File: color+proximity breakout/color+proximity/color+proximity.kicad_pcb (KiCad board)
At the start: 2 copper layers, 72.2 x 21 mm, 59 parts, among them IC1 VL53L4CDV0DH_1, IC2 ISL29125IROZ-T7, J1 RJ12_Shielded, J2 Conn_01x04, J3 Conn_01x06, J8 RJ12_Shielded, J9 Conn_01x06, SW5 SW_Coded_SH-7050, U1 PCA9615DP, U2 LTC4316, U5 TPS73101DBV, U6 ICM-20602

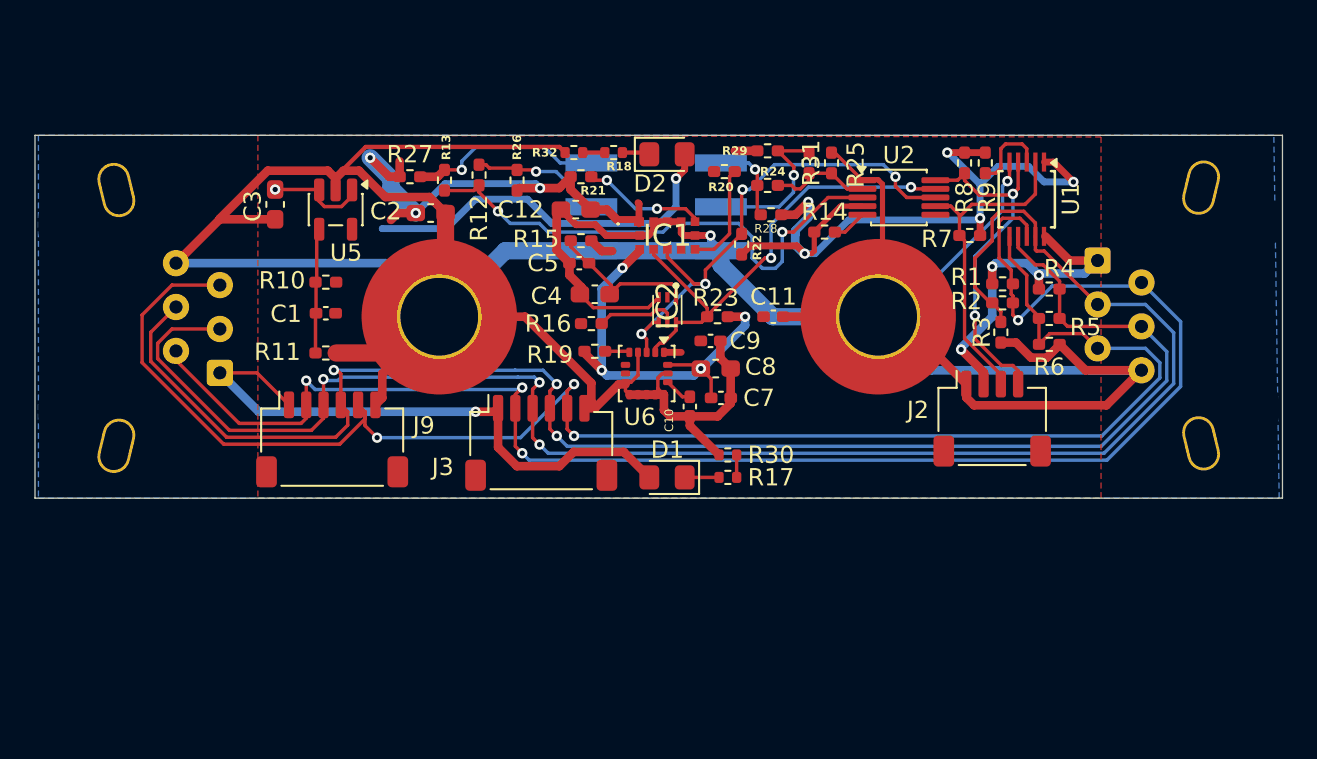
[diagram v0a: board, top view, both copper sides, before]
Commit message: not my finest work but at least it works (i hope)
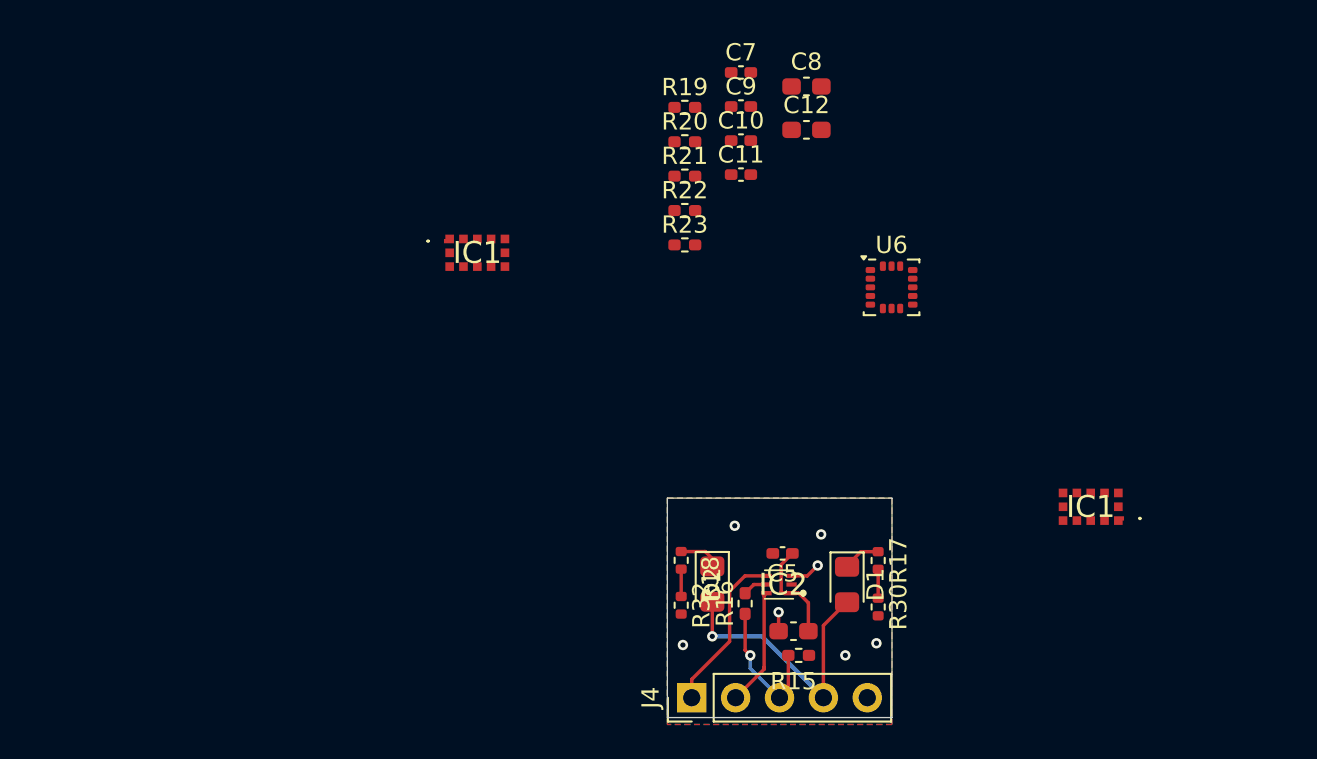
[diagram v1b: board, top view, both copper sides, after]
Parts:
- removed C1: 1n, Capacitor_SMD:C_0402_1005Metric_Pad0.74x0.62mm_HandSolder
- removed C2, C3: 1u, Capacitor_SMD:C_0603_1608Metric_Pad1.08x0.95mm_HandSolder
- removed H1, H2: MountingHole_Pad, MountingHole:MountingHole_4.5mm_Pad_TopOnly
- removed J1, J8: RJ12_Shielded, RJ12_Pin_Connector:RJ12_Pin_Connector
- removed J2: Conn_01x04, Connector_JST:JST_SH_SM04B-SRSS-TB_1x04-1MP_P1.00mm_Horizontal
- removed J3, J9: Conn_01x06, Connector_JST:JST_SH_SM06B-SRSS-TB_1x06-1MP_P1.00mm_Horizontal
- removed R1, R3, R4, R6: 600, Resistor_SMD:R_0402_1005Metric_Pad0.72x0.64mm_HandSolder
- removed R10: 52k, Resistor_SMD:R_0402_1005Metric_Pad0.72x0.64mm_HandSolder
- removed R11: 30k, Resistor_SMD:R_0402_1005Metric_Pad0.72x0.64mm_HandSolder
- removed R12, R24: 400k, Resistor_SMD:R_0402_1005Metric_Pad0.72x0.64mm_HandSolder
- removed R13: 750k, Resistor_SMD:R_0402_1005Metric_Pad0.72x0.64mm_HandSolder
- removed R14, R26, R27, R9: 10k, Resistor_SMD:R_0402_1005Metric_Pad0.72x0.64mm_HandSolder
- removed R2, R5: 120, Resistor_SMD:R_0402_1005Metric_Pad0.72x0.64mm_HandSolder
- removed R25: 780k, Resistor_SMD:R_0402_1005Metric_Pad0.72x0.64mm_HandSolder
- removed R28: 80k, Resistor_SMD:R_0402_1005Metric_Pad0.72x0.64mm_HandSolder
- removed R29: 40k, Resistor_SMD:R_0402_1005Metric_Pad0.72x0.64mm_HandSolder
- removed R31: 260k, Resistor_SMD:R_0402_1005Metric_Pad0.72x0.64mm_HandSolder
- removed R7, R8: 4.7k, Resistor_SMD:R_0402_1005Metric_Pad0.72x0.64mm_HandSolder
- removed SW5: SW_Coded_SH-7050, RJ12_Pin_Connector:Rotary_Switch_16_pos
- removed U1: PCA9615DP, Package_SO:TSSOP-10_3x3mm_P0.5mm
- removed U2: LTC4316, Package_SO:MSOP-10_3x3mm_P0.5mm
- removed U5: TPS73101DBV, Package_TO_SOT_SMD:SOT-23-5
- added IC1: VL53L4CDV0DH_1, VL53L4CD:VL53L4CDV0DH1, F.Cu at (126.2, 105.3)
- added J4: Conn_01x05, Connector_PinHeader_2.54mm:PinHeader_1x05_P2.54mm_Vertical, F.Cu at (103.1, 116.3)
- moved R15 27.1 mm to (109.3, 113.9), turned to 180 degrees
- moved R32 26.9 mm to (102.5, 111.0), turned to -90 degrees
- moved D2 25.0 mm to (104.3, 109.8), turned to -90 degrees
- moved R18 23.9 mm to (102.5, 108.4), turned to -90 degrees
- moved C4 22.6 mm to (109.0, 112.5)
- moved C5 20.5 mm to (108.4, 108.0)
- moved C7 18.9 mm to (106.0, 80.2)
- moved R16 18.5 mm to (106.2, 110.9), turned to 90 degrees
- moved IC2 17.2 mm to (108.2, 109.8), turned to 180 degrees
- moved C8 17.1 mm to (109.8, 81.0)
- moved C10 15.7 mm to (106.0, 84.1), turned to 0 degrees
- moved R19 15.0 mm to (102.7, 82.2)
- moved U6 15.0 mm to (114.7, 92.6), turned to 0 degrees
- moved C12 14.1 mm to (109.8, 83.5), turned to 0 degrees
- moved C9 13.7 mm to (106.0, 82.1)
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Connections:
- IC2 pad 4: /Sensors/sda -> /sda
- IC2 pad 6: /Sensors/scl -> /scl
- R22 pad 2: /Sensors/sda -> /sda
- R23 pad 2: /Sensors/scl -> /scl
- U6 pad 2: /Sensors/scl -> /scl
- U6 pad 3: /Sensors/sda -> /sda
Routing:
- net GND: track 236.8 -> 2.92 mm, vias 2 -> 7
- net Net-(J3-Pin_3): track 98.5 -> 0.00 mm, vias 3 -> 0
- net Net-(J3-Pin_5): track 93.3 -> 0.00 mm, vias 3 -> 0
- net Net-(J3-Pin_2): track 92.6 -> 0.00 mm, vias 4 -> 0
- net Net-(J3-Pin_4): track 89.3 -> 0.00 mm, vias 3 -> 0
- net +3.3V: track 97.1 -> 8.34 mm, vias 12 -> 1
- net +5V: track 82.4 -> 16.0 mm, vias 6 -> 1
- net Net-(U2-XORL): track 30.4 -> 0.00 mm, vias 2 -> 0
- net /Sensors/sda: track 29.9 -> 0.00 mm, vias 4 -> 0
- net /Sensors/scl: track 27.0 -> 0.00 mm, vias 2 -> 0
- net Net-(J2-Pin_4): track 20.8 -> 0.00 mm, vias 2 -> 0
- net Net-(J2-Pin_3): track 19.3 -> 0.00 mm
- net Net-(R13-Pad1): track 11.3 -> 0.00 mm, vias 1 -> 0
- net /sda: track 0.00 -> 9.57 mm
- net Net-(R25-Pad1): track 9.18 -> 0.00 mm, vias 1 -> 0
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- added copper zone on B.Cu, net GND
- added copper zone on F.Cu, net GND
- removed copper zone on F.Cu, net +3.3V
- removed copper zone on B.Cu, net +5V
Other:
- board size 72.2 x 21 mm -> 13 x 12.7 mm
